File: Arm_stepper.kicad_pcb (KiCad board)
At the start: 2 copper layers, 154.5 x 60 mm, 133 parts, among them IC1 L6208D, J1 12V_CONN, J10 ENCODER1, J11 ENCODER2, J3 M1_CONN, J4 Conn_01x06_Male, J5 I2C_CONN, J8 Conn_01x04_Female, J9 USB_B_Mini, M3 MountingHole_3mm, Q2 2N2219, SW1 SW_Push_Dual, SW2 endstop4, SW3 endstop1, SW4 endstop3, SW5 endstop2, U1 ISO1050-00_isolation, U2 USBLC6-2SC6, U3 STM32F446RETx, U4 LM1117-3.3, U5 LM1117-5, Y1 8Mhz

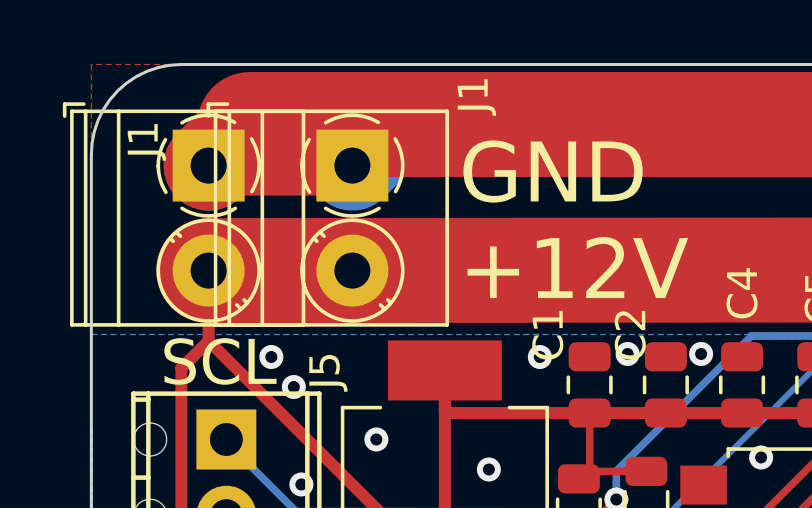
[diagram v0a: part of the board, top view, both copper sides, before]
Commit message: fixx
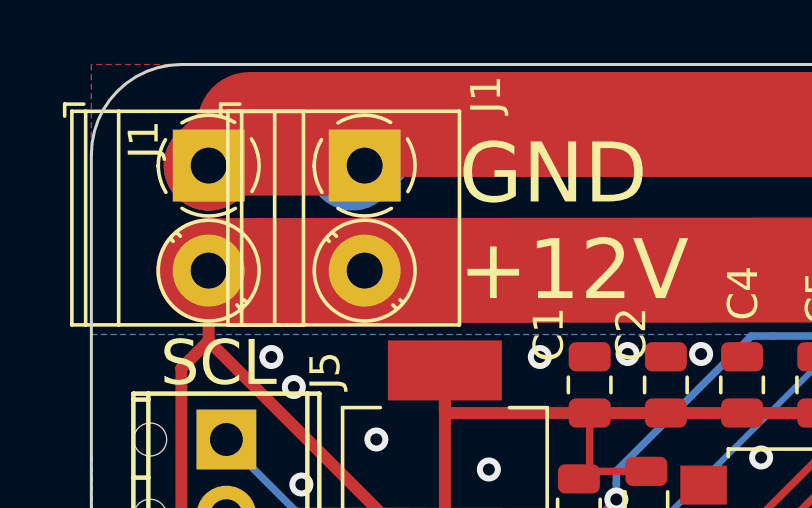
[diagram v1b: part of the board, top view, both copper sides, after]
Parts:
- moved J1 0.41 mm to (47.1, 99.4)
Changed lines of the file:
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@@
   )
   (setup
-    (last_trace_width 3)
+    (last_trace_width 0.25)
     (user_trace_width 0.2)
     (user_trace_width 0.4)
@@
   )
   (module TerminalBlock_Phoenix:TerminalBlock_Phoenix_PT-1,5-2-3.5-H_1x02_P3.50mm_Horizontal (layer F.Cu)
-    (at 46.7 99.37 270)
+    (at 47.11 99.37 270)
     (descr "Terminal Block Phoenix PT-1,5-2-3.5-H, 2 pins, pitch 3.5mm, size 7x7.6mm^2, drill diamater 1.2mm, pad diameter 2.4mm, see , script-generated using https://github.com/pointhi/kicad-footprint-generator/scripts/TerminalBlock_Phoenix")
     (tags "THT Terminal Block Phoenix PT-1,5-2-3.5-H pitch 3.5mm size 7x7.6mm^2 drill 1.2mm pad 2.4mm")
